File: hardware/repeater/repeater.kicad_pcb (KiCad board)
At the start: 2 copper layers, 25.5 x 42 mm, 50 parts, among them J1 Screw_Terminal_01x06, J2 Conn_01x08, J3 Screw_Terminal_01x06, U1 TJA1051T-3, U2 74LVC1G00, U3 74LVC2G74, U6 TJA1051T-3, U8 TD1465

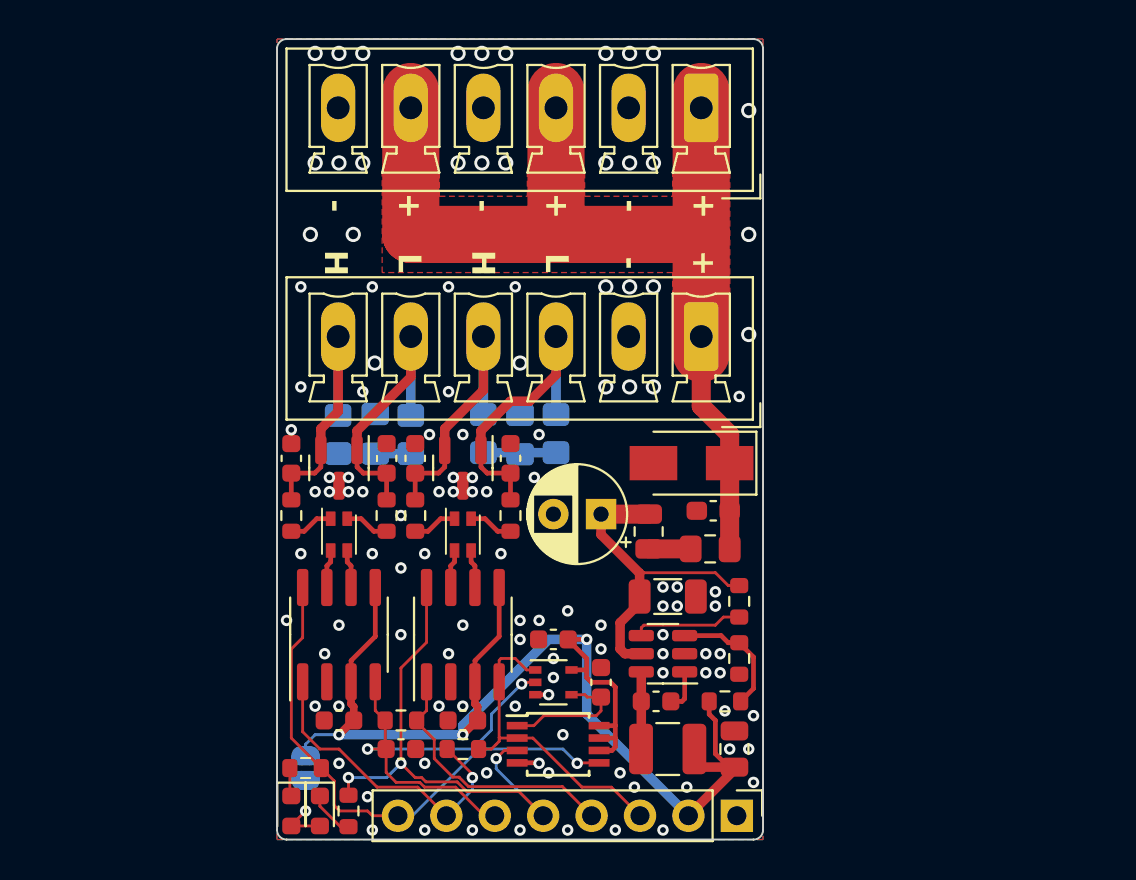
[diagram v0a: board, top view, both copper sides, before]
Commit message: completed repeater
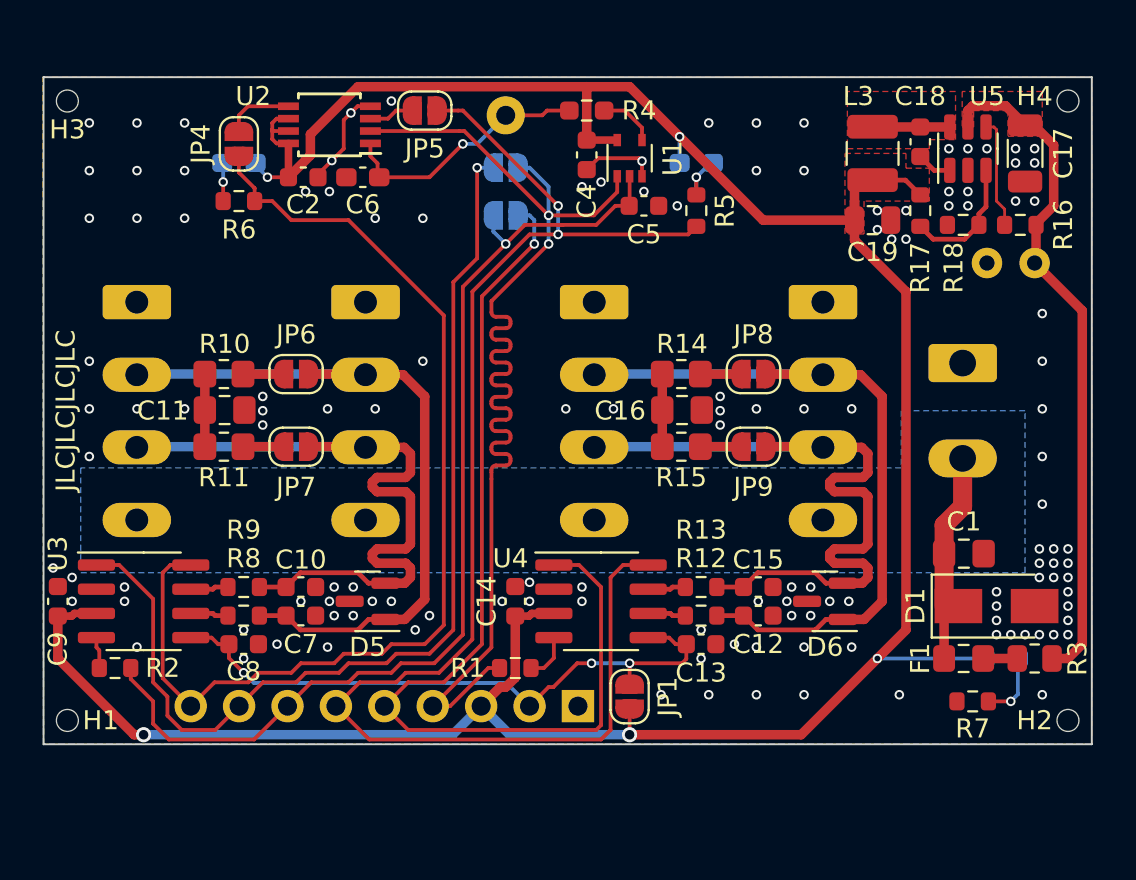
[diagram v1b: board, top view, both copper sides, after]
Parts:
- removed L4, L5: L_Ferrite_Coupled, Inductor_SMD:L_CommonModeChoke_Coilcraft_0805USB
- added C13: 100n, Capacitor_SMD:C_0603_1608Metric, F.Cu at (134.5, 79.8)
- added C4: 100n, Capacitor_SMD:C_0603_1608Metric, F.Cu at (128.5, 54.1)
- added C8: 100n, Capacitor_SMD:C_0603_1608Metric, F.Cu at (110.5, 79.8)
- added D4: LED_P, LED_SMD:LED_0603_1608Metric_Pad1.05x0.95mm_HandSolder, B.Cu at (150.2, 80.5)
- added H1: MountingHole, MountingHole:ToolingHole_1.152mm, F.Cu at (101.2, 83.8)
- added H2: MountingHole, MountingHole:ToolingHole_1.152mm, F.Cu at (153.8, 83.8)
- added H3: MountingHole, MountingHole:ToolingHole_1.152mm, F.Cu at (101.2, 51.2)
- added H4: MountingHole, MountingHole:ToolingHole_1.152mm, F.Cu at (153.8, 51.2)
- added J4: Screw_Terminal_01x04, Connector_Phoenix_MC:PhoenixContact_MCV_1,5_4-G-3.81_1x04_P3.81mm_Vertical, B.Cu at (140.9, 61.8)
- added J5: Screw_Terminal_01x04, Connector_Phoenix_MC:PhoenixContact_MCV_1,5_4-G-3.81_1x04_P3.81mm_Vertical, B.Cu at (104.9, 61.8)
- added J6: Conn_01x09, Connector_PinHeader_2.54mm:PinHeader_1x09_P2.54mm_Vertical, B.Cu at (128.0, 83.0)
- added JP2: Jumper_2_Open, Jumper:SolderJumper-2_P1.3mm_Open_RoundedPad1.0x1.5mm, B.Cu at (124.2, 54.8)
- added JP3: Jumper_2_Open, Jumper:SolderJumper-2_P1.3mm_Open_RoundedPad1.0x1.5mm, B.Cu at (124.2, 57.2)
- added JP4: Jumper_2_Open, Jumper:SolderJumper-2_P1.3mm_Open_RoundedPad1.0x1.5mm, F.Cu at (110.2, 53.5)
- added JP5: Jumper_2_Open, Jumper:SolderJumper-2_P1.3mm_Open_RoundedPad1.0x1.5mm, F.Cu at (120.0, 51.8)
- added JP6: Jumper_2_Open, Jumper:SolderJumper-2_P1.3mm_Open_RoundedPad1.0x1.5mm, F.Cu at (113.2, 65.6)
- added JP7: Jumper_2_Open, Jumper:SolderJumper-2_P1.3mm_Open_RoundedPad1.0x1.5mm, F.Cu at (113.2, 69.4)
- added JP8: Jumper_2_Open, Jumper:SolderJumper-2_P1.3mm_Open_RoundedPad1.0x1.5mm, F.Cu at (137.2, 65.6)
- added JP9: Jumper_2_Open, Jumper:SolderJumper-2_P1.3mm_Open_RoundedPad1.0x1.5mm, F.Cu at (137.2, 69.4)
- added R4: 0, Resistor_SMD:R_0603_1608Metric_Pad0.98x0.95mm_HandSolder, F.Cu at (128.5, 51.8)
- added R7: 1k, Resistor_SMD:R_0603_1608Metric, F.Cu at (148.8, 82.8)
- added TP1: TestPoint, TestPoint:TestPoint_Loop_D1.80mm_Drill1.0mm_Beaded, B.Cu at (124.2, 52.0)
- C1: value C -> 1nF 1kV; footprint Capacitor_SMD:C_0603_1608Metric_Pad1.08x0.95mm_HandSolder -> Capacitor_SMD:C_0805_2012Metric_Pad1.18x1.45mm_HandSolder
- C11: renamed from C14; value C -> 100nF 100V; moved to F.Cu
- C16: renamed from C17; value C -> 100nF 100V; moved to F.Cu
- C3: footprint Capacitor_THT:CP_Radial_D5.0mm_P2.50mm -> Capacitor_THT:C_Disc_D3.0mm_W1.6mm_P2.50mm; moved to B.Cu
- C5: renamed from C12; value 5pF -> 10pF
- C6: renamed from C13; value C -> C_CLK; footprint Capacitor_SMD:C_0603_1608Metric -> Capacitor_SMD:C_0603_1608Metric_Pad1.08x0.95mm_HandSolder
- D1: value D_Zener -> SMAJ24A
- D2: renamed from D4; footprint LED_SMD:LED_0603_1608Metric -> LED_SMD:LED_0603_1608Metric_Pad1.05x0.95mm_HandSolder; moved to B.Cu
- D3: renamed from D5; footprint LED_SMD:LED_0603_1608Metric -> LED_SMD:LED_0603_1608Metric_Pad1.05x0.95mm_HandSolder; moved to B.Cu
- D5: renamed from D6; value SM712_SOT23 -> NUP2105L
- D6: renamed from D7; value SM712_SOT23 -> NUP2105L
- J1: value Screw_Terminal_01x06 -> Screw_Terminal_01x02; footprint Connector_Phoenix_MC:PhoenixContact_MCV_1,5_6-G-3.81_1x06_P3.81mm_Vertical -> Connector_Phoenix_MSTB:PhoenixContact_MSTBA_2,5_2-G_1x02_P5.00mm_Horizontal; moved to B.Cu
- J2: value Conn_01x08 -> Screw_Terminal_01x04; footprint Connector_PinHeader_2.54mm:PinHeader_1x08_P2.54mm_Vertical -> Connector_Phoenix_MC:PhoenixContact_MCV_1,5_4-G-3.81_1x04_P3.81mm_Vertical; moved to B.Cu
- J3: value Screw_Terminal_01x06 -> Screw_Terminal_01x04; footprint Connector_Phoenix_MC:PhoenixContact_MCV_1,5_6-G-3.81_1x06_P3.81mm_Vertical -> Connector_Phoenix_MC:PhoenixContact_MCV_1,5_4-G-3.81_1x04_P3.81mm_Vertical; moved to B.Cu
- JP1: value SolderJumper_2_Open -> Jumper_2_Open; moved to F.Cu
- R1: renamed from R2; value R -> 10
- R10: renamed from R15; value R -> 50; moved to F.Cu
- R11: renamed from R16; value R -> 50; moved to F.Cu
- R12: renamed from R18; value R -> 0
- R13: renamed from R21; value R -> 0
- R14: renamed from R19; value R -> 50; moved to F.Cu
- R15: renamed from R20; value R -> 50; moved to F.Cu
- R17: renamed from R43; value 43k -> 39k
- R18: renamed from R44; value 8k2 -> 7k5
- R2: renamed from R3; value R -> 10
- R3: renamed from R1; value R -> 1
- R5: renamed from R4; value R -> 1k
- R6: renamed from R5; value R -> 1k
- R8: renamed from R14; value R -> 0
- R9: renamed from R17; value R -> 0
- moved D2 39.3 mm to (134.2, 54.5), turned to 180 degrees
- moved R5 36.4 mm to (134.2, 57.0), turned to -90 degrees
- moved U2 34.6 mm to (115.0, 52.5), turned to 180 degrees
- moved D3 34.1 mm to (110.2, 54.5), turned to 0 degrees
- moved L3 33.0 mm to (143.5, 54.0), turned to -90 degrees
- moved C18 32.5 mm to (146.0, 53.4), turned to 90 degrees
- moved C5 31.2 mm to (131.5, 56.8)
- moved U5 31.0 mm to (148.5, 53.8), turned to 90 degrees
- moved R6 30.0 mm to (110.2, 56.5)
- moved C17 29.9 mm to (151.5, 54.0), turned to 90 degrees
- moved C6 29.3 mm to (116.8, 55.2), turned to 180 degrees
- moved C19 28.7 mm to (143.5, 57.5), turned to 180 degrees
- moved J2 28.0 mm to (128.9, 61.8)
- moved U1 27.8 mm to (130.8, 54.2), turned to 90 degrees
- moved R17 27.7 mm to (146.0, 57.0), turned to -90 degrees
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- renumbered C15 to C10, C16 to C12, C26 to C14, C18 to C15, C40 to C17, C41 to C18, C42 to C19, C11 to C2, C2 to C7, C7 to C9, L2 to L3, R42 to R16, U2 to U1, U3 to U2, U1 to U3, U6 to U4, U8 to U5
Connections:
- net /XCVR/CAN_{SPLIT} renamed /XCVR0/CAN_{SPLIT}
- D2 pad 2: +5VL -> +5V
- D3 pad 2: +5VL -> +5V
- J1 pad 1: VBUS -> GND
- J1 pad 2: GND -> VBUS
- J2 pad 2: +5V -> /L_0
- J2 pad 3: /RX_0 -> /H_0
- J2 pad 4: /TX_0 -> VBUS
- J3 pad 1: VBUS -> GND
- J3 pad 2: GND -> /L_1
- J3 pad 3: VBUS -> /H_1
- J3 pad 4: GND -> VBUS
- JP1 pad 2: +5VL -> /VIO
- R1 pad 1: /RX_0 -> /XCVR0/RX_{CAN}
- R1 pad 2: /TX_1 -> /RX_0
- R10 pad 1: /L_1 -> Net-(JP6-B)
- R11 pad 2: /H_1 -> Net-(JP7-A)
- R12 pad 2: Net-(L5-Pad4) -> /XCVR0/L
- R13 pad 2: Net-(L5-Pad1) -> /XCVR0/H
- R14 pad 1: /L_0 -> Net-(JP8-B)
- R15 pad 2: /H_0 -> Net-(JP9-A)
- R2 pad 1: /RX_1 -> /XCVR1/RX_{CAN}
- R2 pad 2: /TX_0 -> /RX_1
- R8 pad 2: Net-(L4-Pad4) -> /XCVR1/L
- R9 pad 2: Net-(L4-Pad1) -> /XCVR1/H
- U1 pad 4: /CLK -> /C
- U2 pad 3: /S_0 -> /~{Q}
- U2 pad 5: /S_1 -> /Q
- U3 pad 4: /RX_1 -> /XCVR1/RX_{CAN}
- U3 pad 5: +5V -> /VIO
- U4 pad 4: /RX_0 -> /XCVR0/RX_{CAN}
- U4 pad 5: +5V -> /VIO
- U4 pad 6: /XCVR/L -> /XCVR0/L
- U4 pad 7: /XCVR/H -> /XCVR0/H
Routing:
- net +5V: track 68.9 -> 146.6 mm, vias 3 -> 5
- net /S_0: track 27.7 -> 75.5 mm, vias 3 -> 2
- net /RX_0: track 16.8 -> 63.1 mm, vias 0 -> 2
- net VBUS: track 55.8 -> 11.4 mm
- net /TX_0: track 14.1 -> 53.0 mm, vias 0 -> 1
- net /TX_1: track 16.6 -> 53.3 mm
- net /VIO: track 0.00 -> 33.0 mm, vias 0 -> 3
- net /RX_1: track 23.3 -> 54.6 mm, vias 2 -> 1
- net /S_1: track 28.5 -> 55.6 mm, vias 1 -> 0
- net /H_1: track 14.4 -> 39.4 mm
- net /H_0: track 14.9 -> 39.4 mm
- net /L_1: track 15.2 -> 38.9 mm
- net /L_0: track 16.2 -> 38.9 mm
- net +24V: track 19.0 -> 35.8 mm
- net GND: track 1.86 -> 9.27 mm, vias 117 -> 134
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- added copper zone on F.Cu, net +24V
- added copper zone on F.Cu, net +5V
- added copper zone on F.Cu, net /vreg/SW
- added copper zone on B.Cu, net VBUS
- removed copper zone on F.Cu, net VBUS
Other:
- board size 25.5 x 42 mm -> 55 x 35 mm
- board text added: "-+"
- board text added: "0 Active"
- board text added: "1 Active"
- board text added: "BUS repeater"
- board text added: "JLCJLCJLCJLC"
- board text added: "L H"
- board text added: "Power"
- board text added: "S_1 TX1 RX1 S_0 TX0 RX0 +5V VIO GND"
- board text removed: "+ - + - + -"
- board text removed: "+ - L H L H"
- board text removed: "CAN BUS repeater"
- board text removed: "GND +5V RX0 TX0 S_0 RX1 TX1 S_1"
- board text removed: "LED_EN"
